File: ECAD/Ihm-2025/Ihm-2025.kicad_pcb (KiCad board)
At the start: 2 copper layers, 58 x 58 mm, 23 parts, among them SW1 SW_SPDT, SW2 SW_SPDT, SW3 SW_SPDT, SW4 SW_SPDT

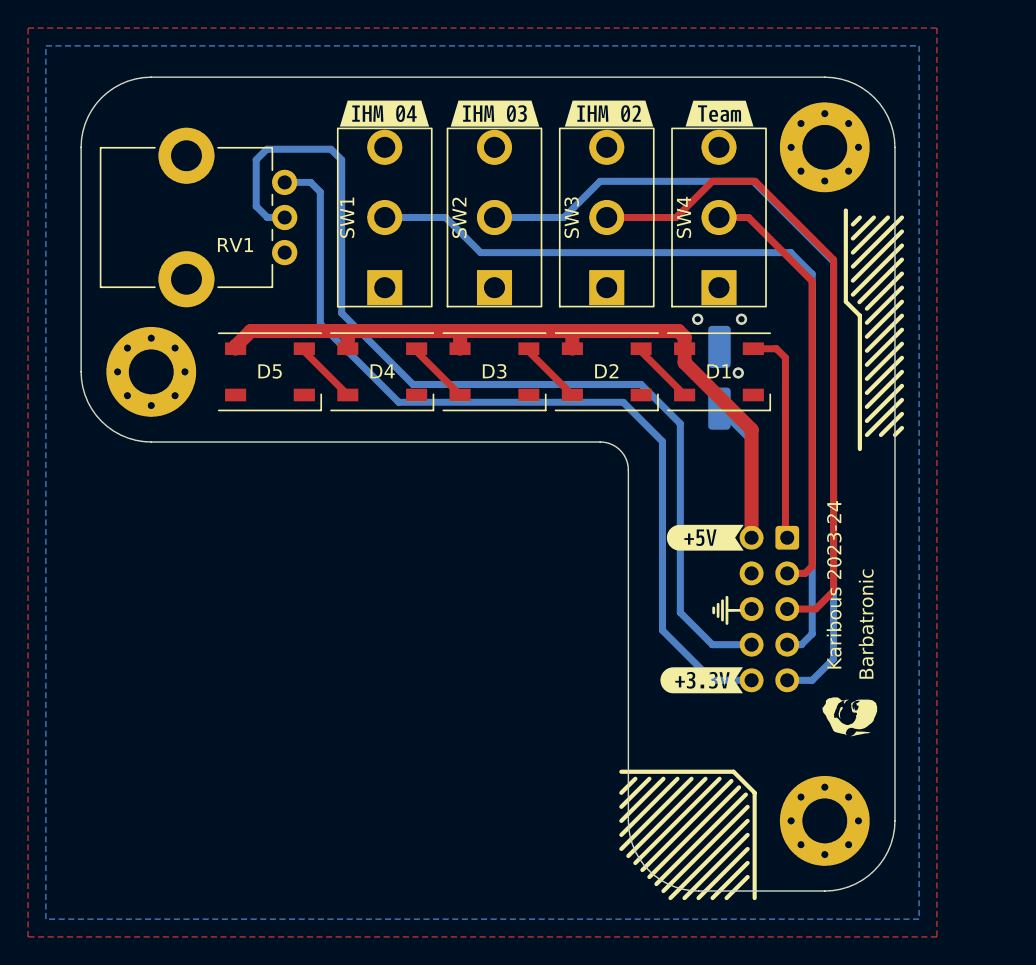
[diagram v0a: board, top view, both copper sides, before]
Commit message: New IHM
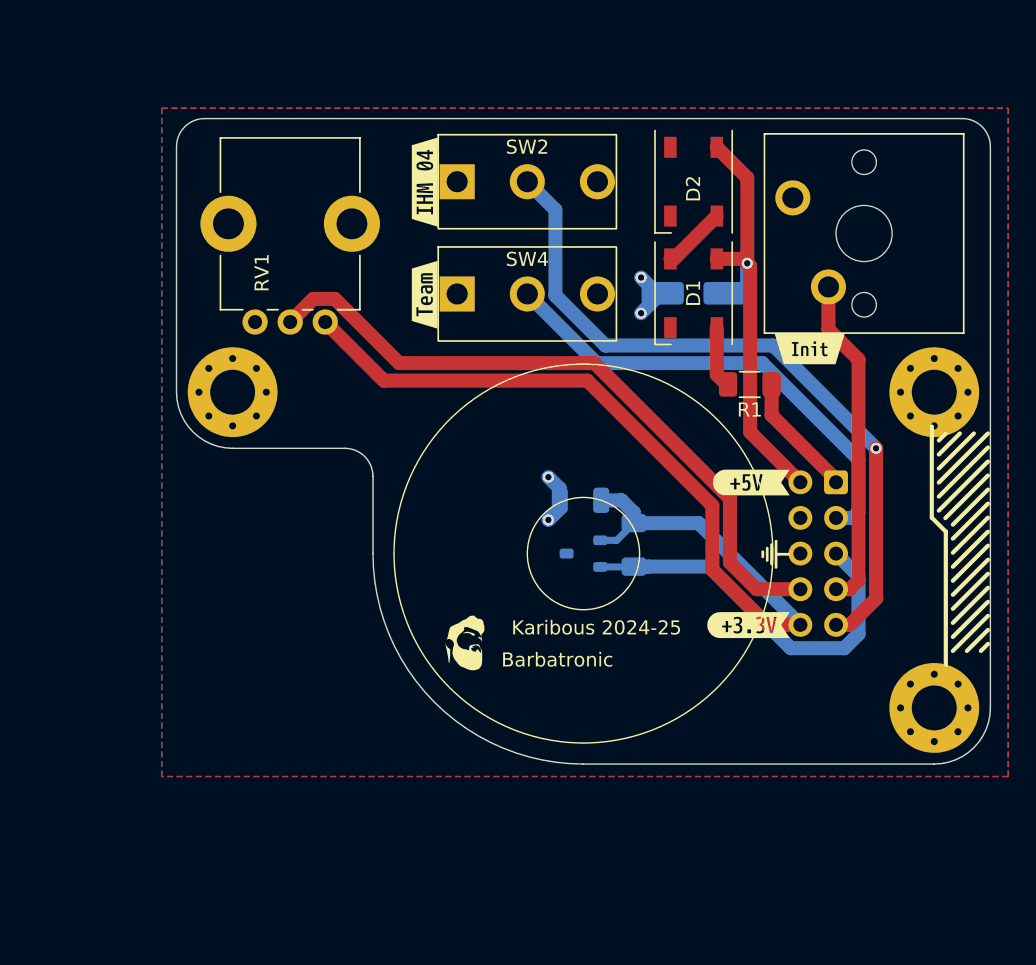
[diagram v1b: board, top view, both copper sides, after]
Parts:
- removed D3, D4, D5: WS2812B, LED_SMD:LED_WS2812B_PLCC4_5.0x5.0mm_P3.2mm
- removed H1: M3, MountingHole:MountingHole_3.2mm_M3_Pad_Via
- removed SW3: SW_SPDT, footprints:SK-12D10 1P2T
- removed kibuzzard-64A1DFBF: G***, kibuzzard-64A1DFBF
- removed kibuzzard-64A1DFD1: G***, kibuzzard-64A1DFD1
- added C2: 100n, Capacitor_SMD:C_1206_3216Metric, B.Cu at (148.6, 97.2)
- added G***: LOGO, LOGO, B.Cu at (155.4, 107.2)
- added H2: M3, MountingHole:MountingHole_3.2mm_M3_Pad_Via, F.Cu at (173.8, 89.5)
- added R1: R_Small, Resistor_SMD:R_1206_3216Metric_Pad1.30x1.75mm_HandSolder, F.Cu at (160.7, 88.9)
- added R2: 4.8k, Resistor_SMD:R_1206_3216Metric_Pad1.30x1.75mm_HandSolder, B.Cu at (152.4, 100.3)
- added U1: ~, Package_TO_SOT_SMD:SOT-23W, B.Cu at (148.8, 101.0)
- added kibuzzard-666F551A: G***, kibuzzard-666F551A, F.Cu at (164.9, 86.4)
- SW1: value SW_SPDT -> SW_Push; footprint footprints:SK-12D10 1P2T -> PCM_Switch_Keyboard_Cherry_MX:SW_Cherry_MX_PCB_1.00u
- moved H3 52.1 mm to (123.8, 89.5)
- moved H4 40.7 mm to (173.8, 112.0)
- moved SW1 34.2 mm to (168.8, 78.1)
- moved G*** 28.0 mm to (140.3, 107.3), turned to 0 degrees
- moved kibuzzard-64A1DFA1 24.7 mm to (137.5, 82.5), turned to 90 degrees
- moved D2 14.9 mm to (156.7, 74.5), turned to -90 degrees
- moved SW4 14.7 mm to (144.8, 82.5), turned to 0 degrees
- moved RV1 10.4 mm to (130.4, 84.5), turned to 90 degrees
- moved C1 6.30 mm to (156.7, 82.4), turned to 180 degrees
- moved D1 5.89 mm to (156.7, 82.4), turned to -90 degrees
- moved kibuzzard-64A1DFD6 5.67 mm to (137.5, 74.5), turned to 90 degrees
- moved G*** 5.32 mm to (162.5, 101.0)
- moved IHM-IO1 5.26 mm to (166.8, 95.9)
- moved kibuzzard-64A1DF73 5.16 mm to (160.6, 106.0)
- moved kibuzzard-64A1DF46 5.13 mm to (160.8, 95.9)
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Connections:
- net DAC0 renamed Analog0
- net DAC1 renamed Analog1
- D1 pad 4: NEO_PIXEL -> Net-(D1-DIN)
- D2 pad 2: Net-(D2-DOUT) -> unconnected-(D2-DOUT-Pad2)
- IHM-IO1 pad 5: Detection -> Tirette
- IHM-IO1 pad 7: IHM_3 -> Init
- SW1 pad 1: GND -> Init
- SW1 pad 2: IHM_3 -> GND
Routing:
- net IHM_3: track 59.9 -> 0.00 mm
- net Detection: track 47.0 -> 0.00 mm
- net +5V: track 63.2 -> 32.4 mm, vias 0 -> 1
- net Tirette: track 0.00 -> 28.7 mm
- net Init: track 0.00 -> 23.7 mm
- net Analog0: track 70.2 -> 48.3 mm
- net IHM_4: track 59.9 -> 50.7 mm, vias 0 -> 1
- net GND: track 0.00 -> 7.86 mm, vias 3 -> 4
- net NEO_PIXEL: track 15.4 -> 8.87 mm
- net +3V3: track 61.4 -> 66.7 mm
- net Net-(D4-DOUT): track 4.58 -> 0.00 mm
- net Net-(D3-DOUT): track 4.58 -> 0.00 mm
- net Net-(D2-DOUT): track 4.58 -> 0.00 mm
- net Net-(D1-DIN): track 0.00 -> 4.44 mm
- net Couleur: track 30.8 -> 34.0 mm
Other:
- board size 58 x 58 mm -> 58 x 46 mm
- board text added: "Karibous 2024-25"
- board text removed: "Karibous 2023-24"
